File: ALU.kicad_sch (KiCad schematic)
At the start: 0 parts

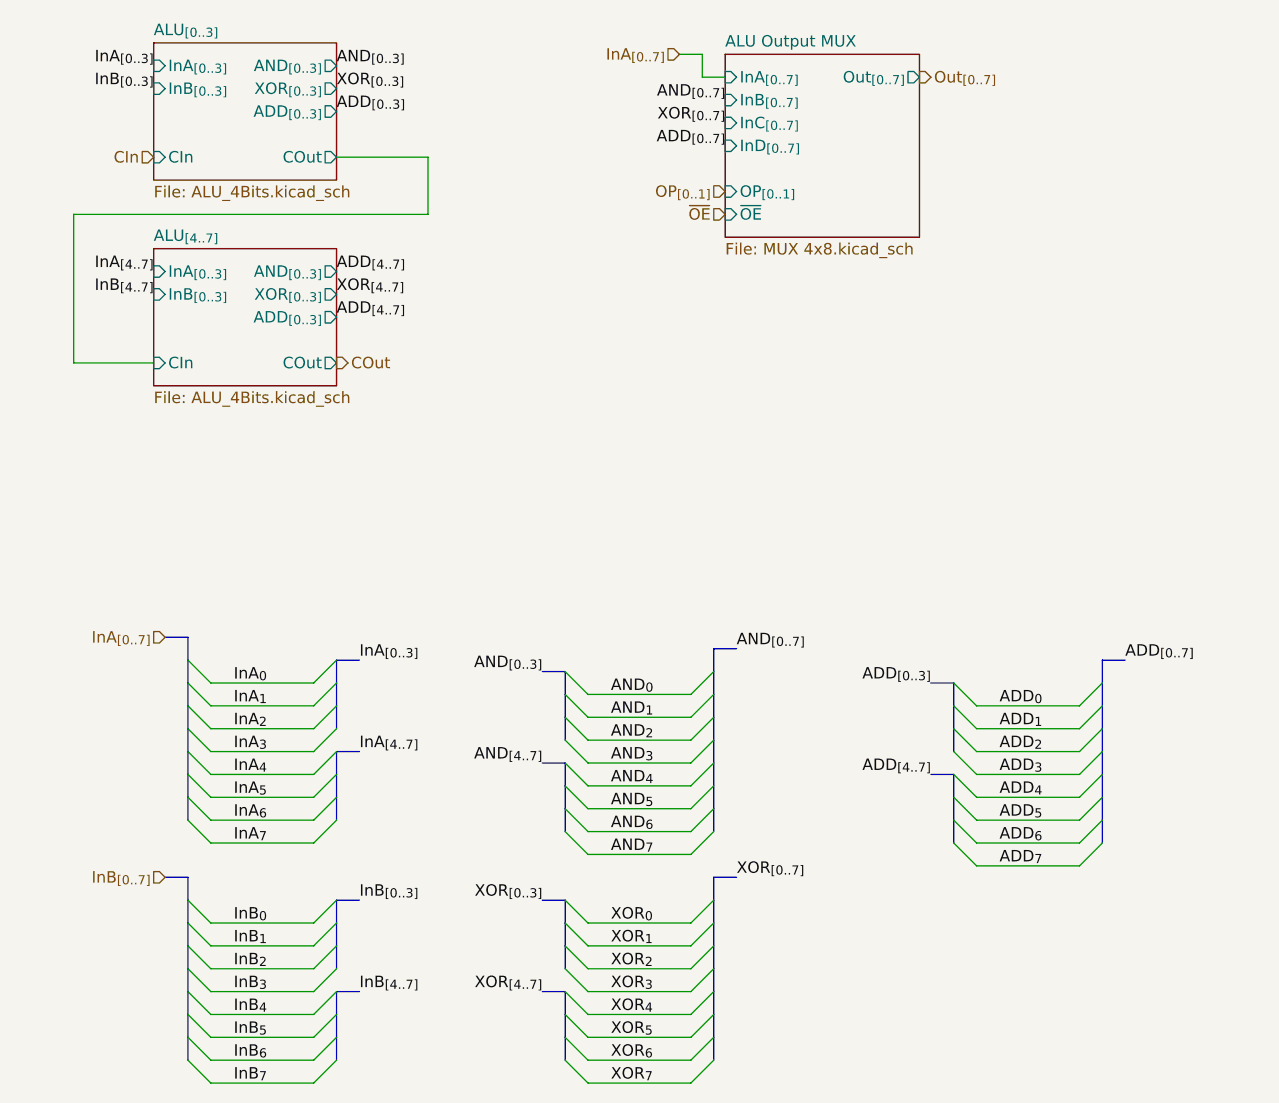
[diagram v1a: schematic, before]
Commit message: Fixed(?)
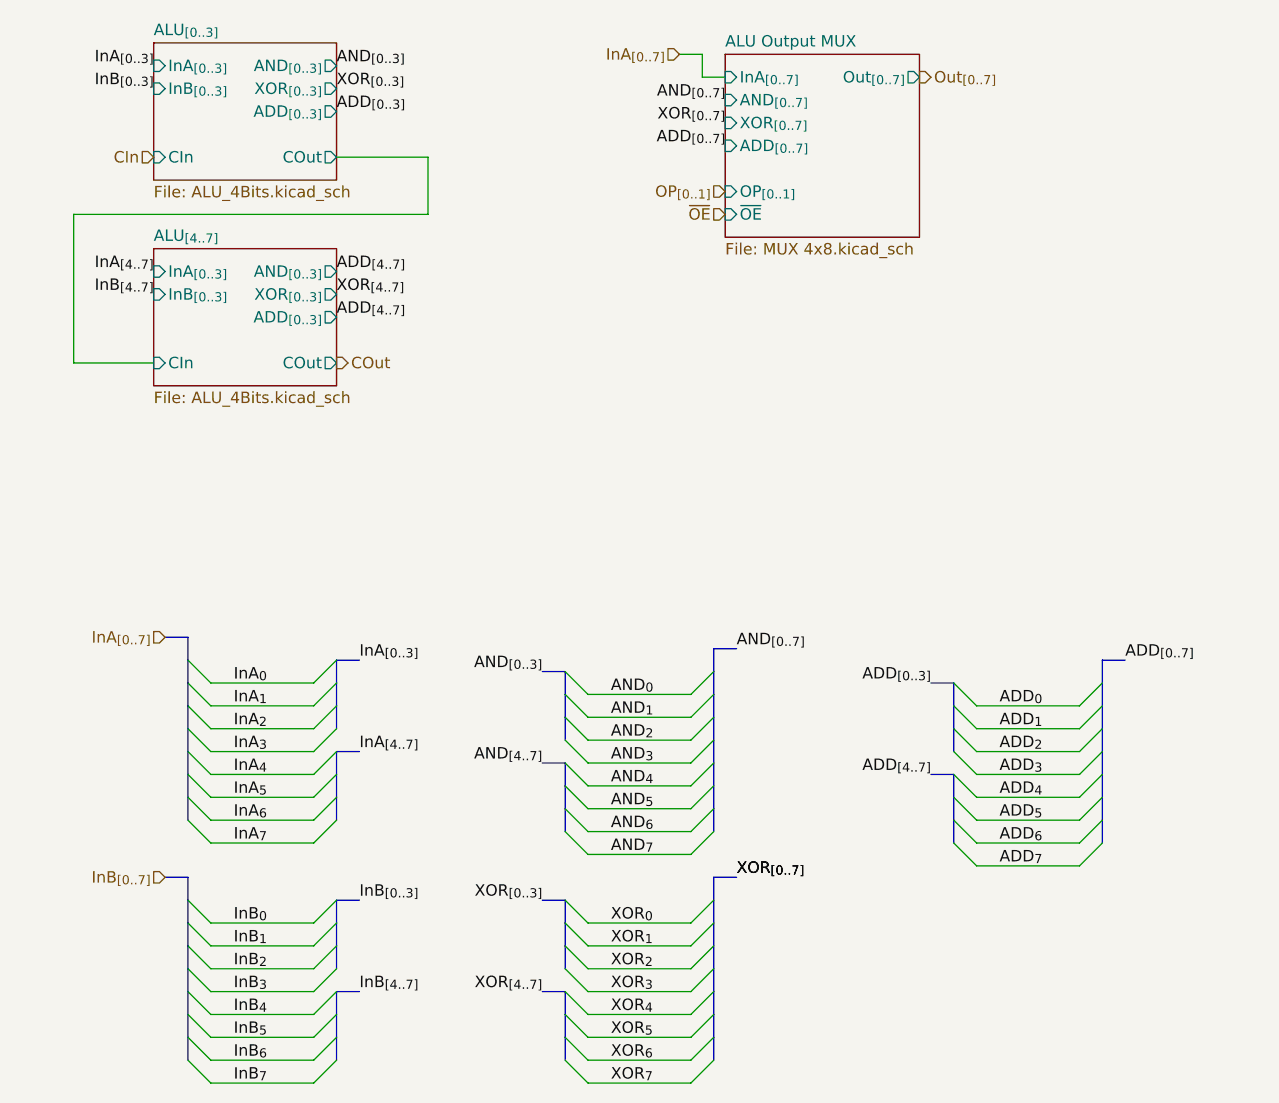
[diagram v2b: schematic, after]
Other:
- sheet ALU Output MUX ports: added ADD_{[0..7]}, AND_{[0..7]}, XOR_{[0..7]}; removed InB_{[0..7]}, InC_{[0..7]}, InD_{[0..7]}
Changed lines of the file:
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@@
+		)
+	)
+	(label "XOR_{2}"
+		(at 92.71 133.35 0)
+		(effects
+			(font
+				(size 1.27 1.27)
+			)
+			(justify left bottom)
+		)
+	)
+	(label "InB_{7}"
+		(at 50.8 146.05 0)
+		(effects
+			(font
+				(size 1.27 1.27)
+			)
+			(justify left bottom)
+		)
+	)
+	(label "AND_{[0..7]}"
+		(at 106.68 97.79 0)
+		(effects
+			(font
+				(size 1.27 1.27)
+			)
+			(justify left bottom)
+		)
+	)
+	(label "InB_{6}"
+		(at 50.8 143.51 0)
+		(effects
+			(font
+				(size 1.27 1.27)
+			)
+			(justify left bottom)
+		)
+	)
+	(label "ADD_{[0..3]}"
+		(at 128.27 101.6 180)
+		(effects
+			(font
+				(size 1.27 1.27)
+			)
+			(justify right bottom)
+		)
+	)
+	(label "XOR_{[4..7]}"
+		(at 85.09 135.89 180)
+		(effects
+			(font
+				(size 1.27 1.27)
+			)
+			(justify right bottom)
+		)
+	)
+	(label "AND_{1}"
+		(at 92.71 105.41 0)
+		(effects
+			(font
+				(size 1.27 1.27)
+			)
+			(justify left bottom)
+		)
+	)
+	(label "ADD_{3}"
+		(at 135.89 111.76 0)
+		(effects
+			(font
+				(size 1.27 1.27)
+			)
+			(justify left bottom)
 		)
 	)
@@
 		)
 	)
-	(label "XOR_{2}"
-		(at 92.71 133.35 0)
-		(effects
-			(font
-				(size 1.27 1.27)
-			)
-			(justify left bottom)
-		)
-	)
-	(label "InB_{7}"
-		(at 50.8 146.05 0)
-		(effects
-			(font
-				(size 1.27 1.27)
-			)
-			(justify left bottom)
-		)
-	)
-	(label "AND_{[0..7]}"
-		(at 106.68 97.79 0)
-		(effects
-			(font
-				(size 1.27 1.27)
-			)
-			(justify left bottom)
-		)
-	)
-	(label "InB_{6}"
-		(at 50.8 143.51 0)
-		(effects
-			(font
-				(size 1.27 1.27)
-			)
-			(justify left bottom)
-		)
-	)
-	(label "ADD_{[0..3]}"
-		(at 128.27 101.6 180)
-		(effects
-			(font
-				(size 1.27 1.27)
-			)
-			(justify right bottom)
-		)
-	)
-	(label "XOR_{[4..7]}"
-		(at 85.09 135.89 180)
-		(effects
-			(font
-				(size 1.27 1.27)
-			)
-			(justify right bottom)
-		)
-	)
-	(label "AND_{1}"
-		(at 92.71 105.41 0)
-		(effects
-			(font
-				(size 1.27 1.27)
-			)
-			(justify left bottom)
-		)
-	)
-	(label "ADD_{3}"
-		(at 135.89 111.76 0)
-		(effects
-			(font
-				(size 1.27 1.27)
-			)
-			(justify left bottom)
-		)
-	)
 	(label "InA_{7}"
 		(at 50.8 119.38 0)
@@
 	(label "XOR_{5}"
 		(at 92.71 140.97 0)
+		(effects
+			(font
+				(size 1.27 1.27)
+			)
+			(justify left bottom)
+		)
+	)
+	(label "XOR_{[0..7]}"
+		(at 106.68 123.19 0)
 		(effects
 			(font
@@
 			)
 		)
-		(pin "InD_{[0..7]}" input
-			(at 105.41 41.91 180)
-			(effects
-				(font
-					(size 1.27 1.27)
-				)
-				(justify left)
-			)
-		)
 		(pin "InA_{[0..7]}" input
 			(at 105.41 34.29 180)
@@
 			)
 		)
-		(pin "InC_{[0..7]}" input
-			(at 105.41 39.37 180)
-			(effects
-				(font
-					(size 1.27 1.27)
-				)
-				(justify left)
-			)
-		)
 		(pin "~{OE}" input
 			(at 105.41 49.53 180)
@@
 			)
 		)
-		(pin "InB_{[0..7]}" input
-			(at 105.41 36.83 180)
-			(effects
-				(font
-					(size 1.27 1.27)
-				)
-				(justify left)
-			)
-		)
 		(pin "OP_{[0..1]}" input
 			(at 105.41 46.99 180)
 			(effects
 				(font
+					(size 1.27 1.27)
+				)
+				(justify left)
+			)
+		)
+		(pin "AND_{[0..7]}" input
+			(at 105.41 36.83 180)
+			(effects
+				(font
+					(size 1.27 1.27)
+				)
+				(justify left)
+			)
+		)
+		(pin "ADD_{[0..7]}" input
+			(at 105.41 41.91 180)
+			(effects
+				(font
+					(size 1.27 1.27)
+				)
+				(justify left)
+			)
+		)
+		(pin "XOR_{[0..7]}" input
+			(at 105.41 39.37 180)
+			(effects
+				(font
